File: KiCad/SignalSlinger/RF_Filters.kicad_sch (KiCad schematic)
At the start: 11 parts, among them J301 To Antenna

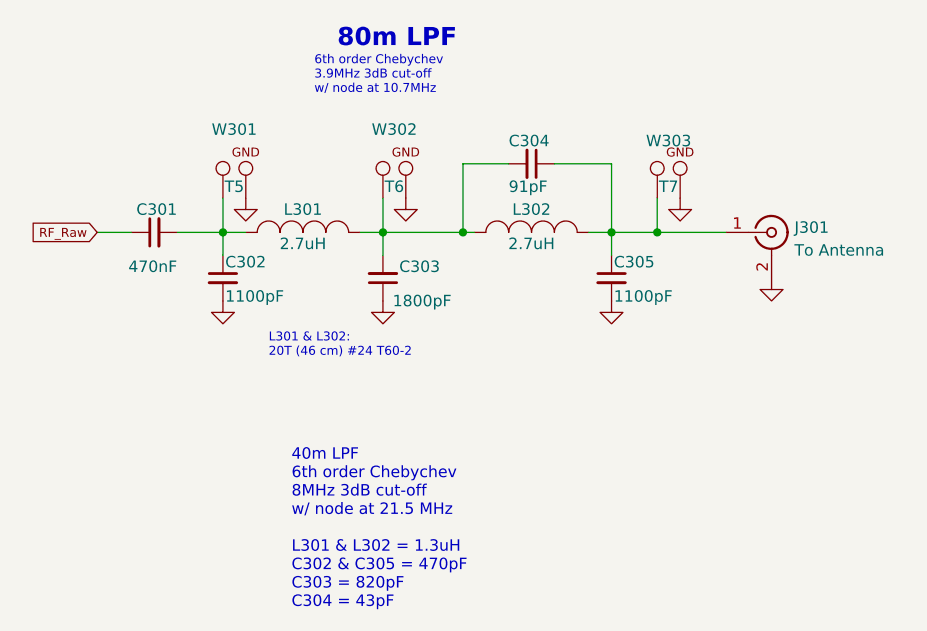
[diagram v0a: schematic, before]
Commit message: Production Updates
Corrects copper spacing issues
Removes warnings
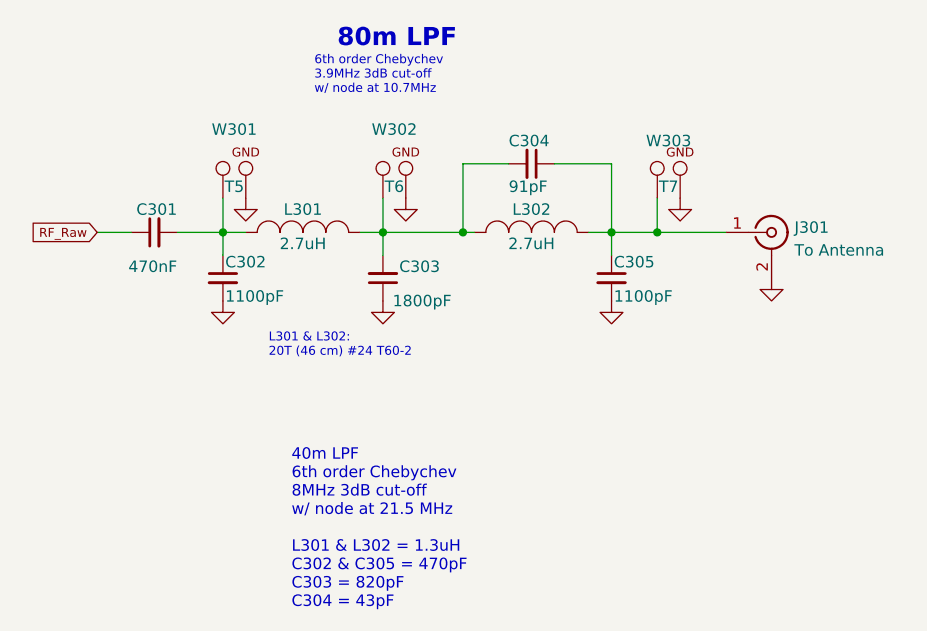
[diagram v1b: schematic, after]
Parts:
- J301: symbol Connector:Conn_Coaxial -> SignalSlinger Library:Conn_Coaxial
- L301, L302: footprint Inductors:Toroid_T-60_2TH_Vertical -> SignalSlinger_Footprints:Toroid_T-60_2TH_Vertical; symbol Device:INDUCTOR_SMALL -> SignalSlinger Library:INDUCTOR_SMALL
- W301, W302, W303: footprint Measurement:Measurement_Point_ScopeProbe_Round-SMD-2sides-Pad_Small -> SignalSlinger_Footprints:Measurement_Point_ScopeProbe_Round-SMD-2sides-Pad_Small; symbol Connector:TEST_SCOPE -> SignalSlinger Library:TEST_SCOPE
